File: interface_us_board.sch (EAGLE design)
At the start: 38 parts, among them IC1 74AC245DW, IC2 4050D

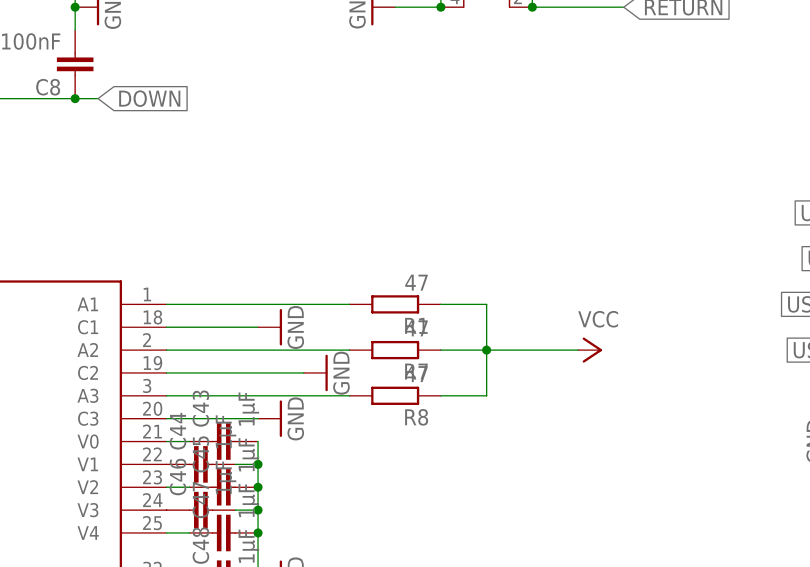
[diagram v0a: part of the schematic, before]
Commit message: InterfaceUSBoard: change resistor value
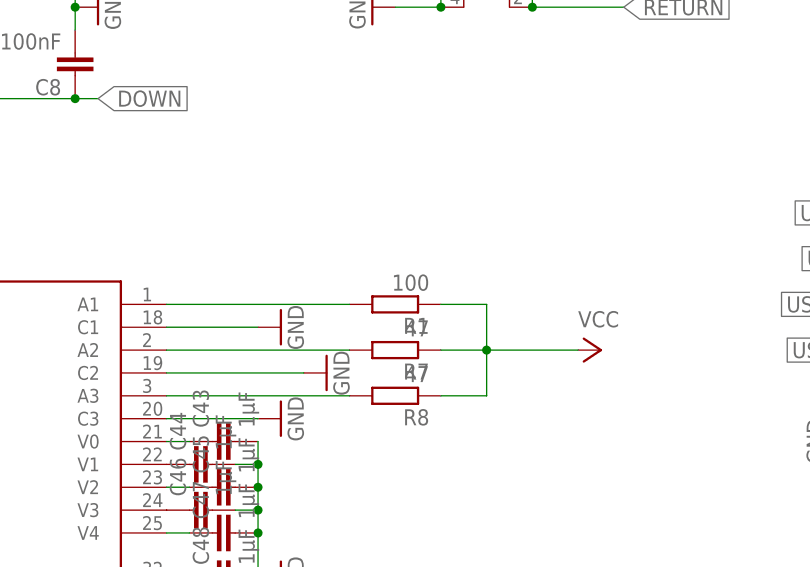
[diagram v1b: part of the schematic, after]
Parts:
- R1: value 47 -> 100
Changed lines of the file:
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@@
 <part name="GND2" library="supply1" deviceset="GND" device=""/>
 <part name="P+1" library="supply1" deviceset="VCC" device=""/>
-<part name="R1" library="resistor" deviceset="R-EU_" device="M1206" value="47"/>
+<part name="R1" library="resistor" deviceset="R-EU_" device="M1206" value="100"/>
 <part name="IC1" library="74xx-eu" deviceset="74*245" device="DW" technology="AC"/>
 <part name="IC2" library="40xx" deviceset="4050" device="D"/>

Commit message: Revert "InterfaceUSBoard: change resistor value" change was not needed
This reverts commit 6388b83db6797b02bafabf1e9fd2be2e5c524c07.
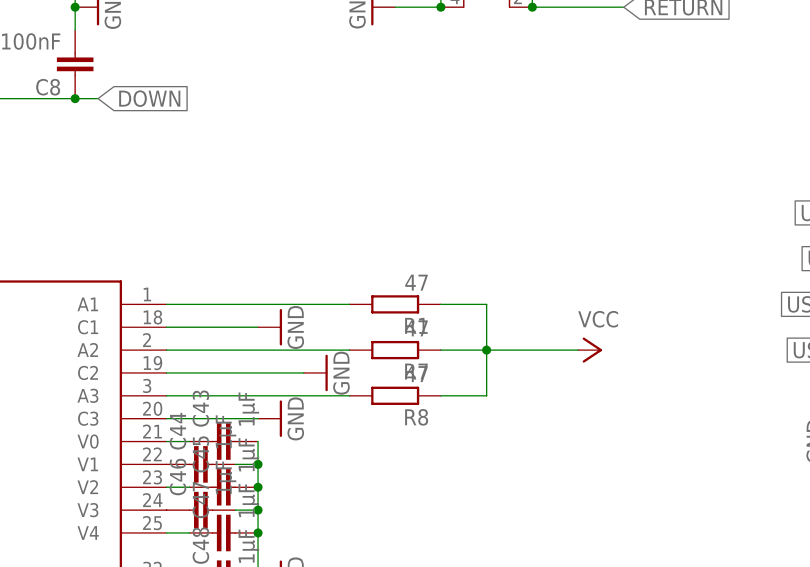
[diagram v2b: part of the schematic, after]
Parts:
- R1: value 100 -> 47
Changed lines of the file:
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@@
 <part name="GND2" library="supply1" deviceset="GND" device=""/>
 <part name="P+1" library="supply1" deviceset="VCC" device=""/>
-<part name="R1" library="resistor" deviceset="R-EU_" device="M1206" value="100"/>
+<part name="R1" library="resistor" deviceset="R-EU_" device="M1206" value="47"/>
 <part name="IC1" library="74xx-eu" deviceset="74*245" device="DW" technology="AC"/>
 <part name="IC2" library="40xx" deviceset="4050" device="D"/>
